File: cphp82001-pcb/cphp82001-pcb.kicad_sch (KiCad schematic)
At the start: 32 parts, among them J1 USB_B_Micro, J2 PAD+, J3 PAD-, Q1 2N7002, U1 BQ21040, U2 TLV75801, U3 MAX40203AUK, U4 TPS3808DBV, U6 NCP360SNT

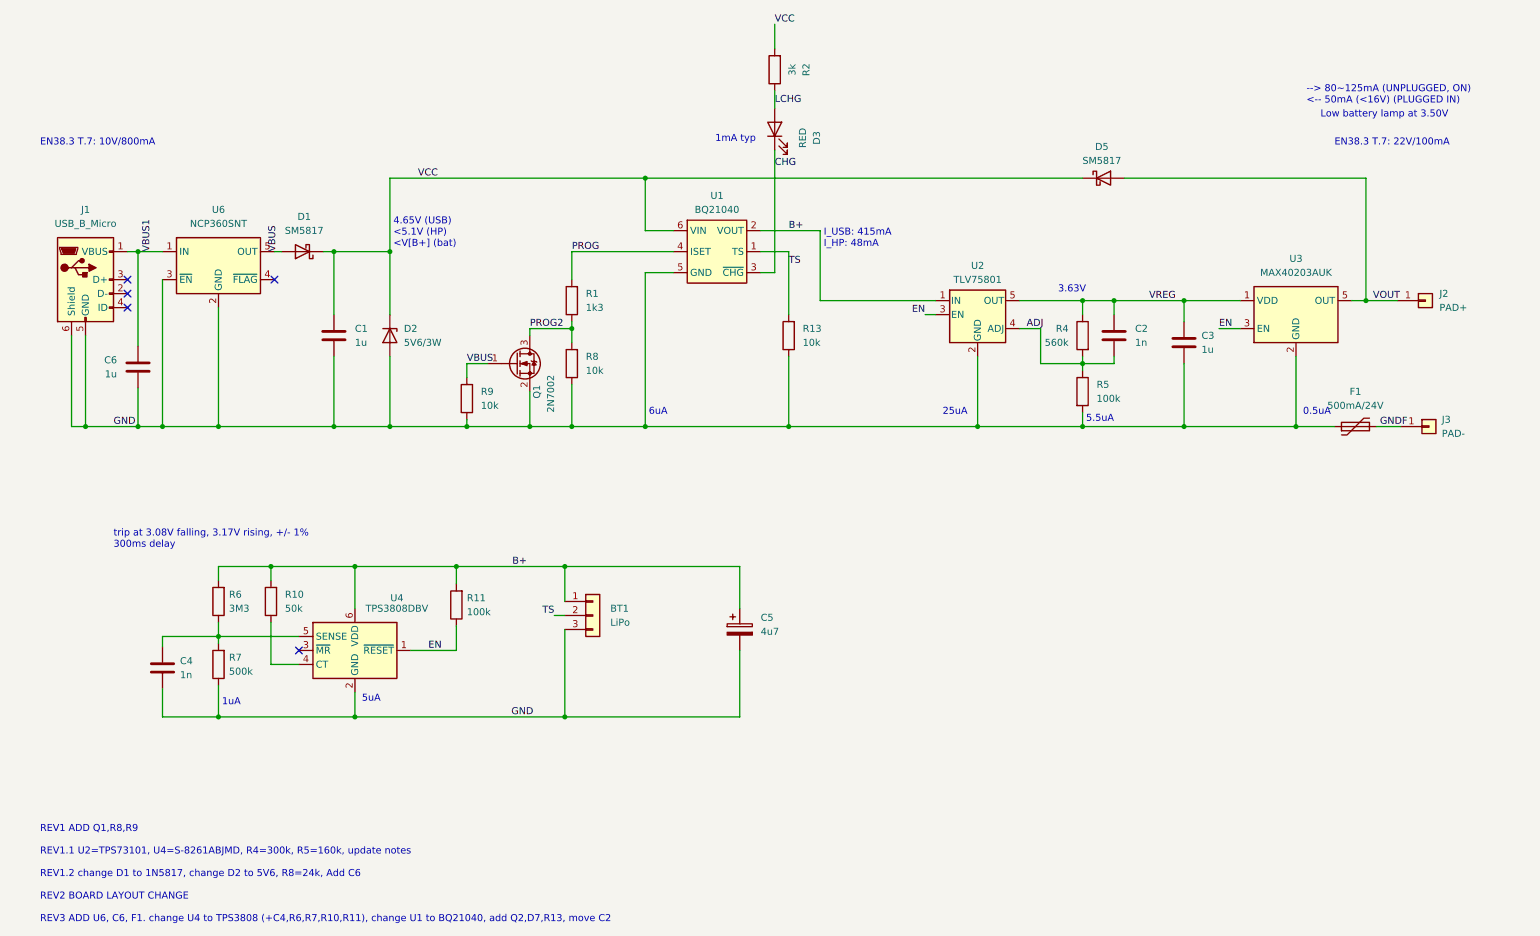
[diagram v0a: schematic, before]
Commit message: Update rev3
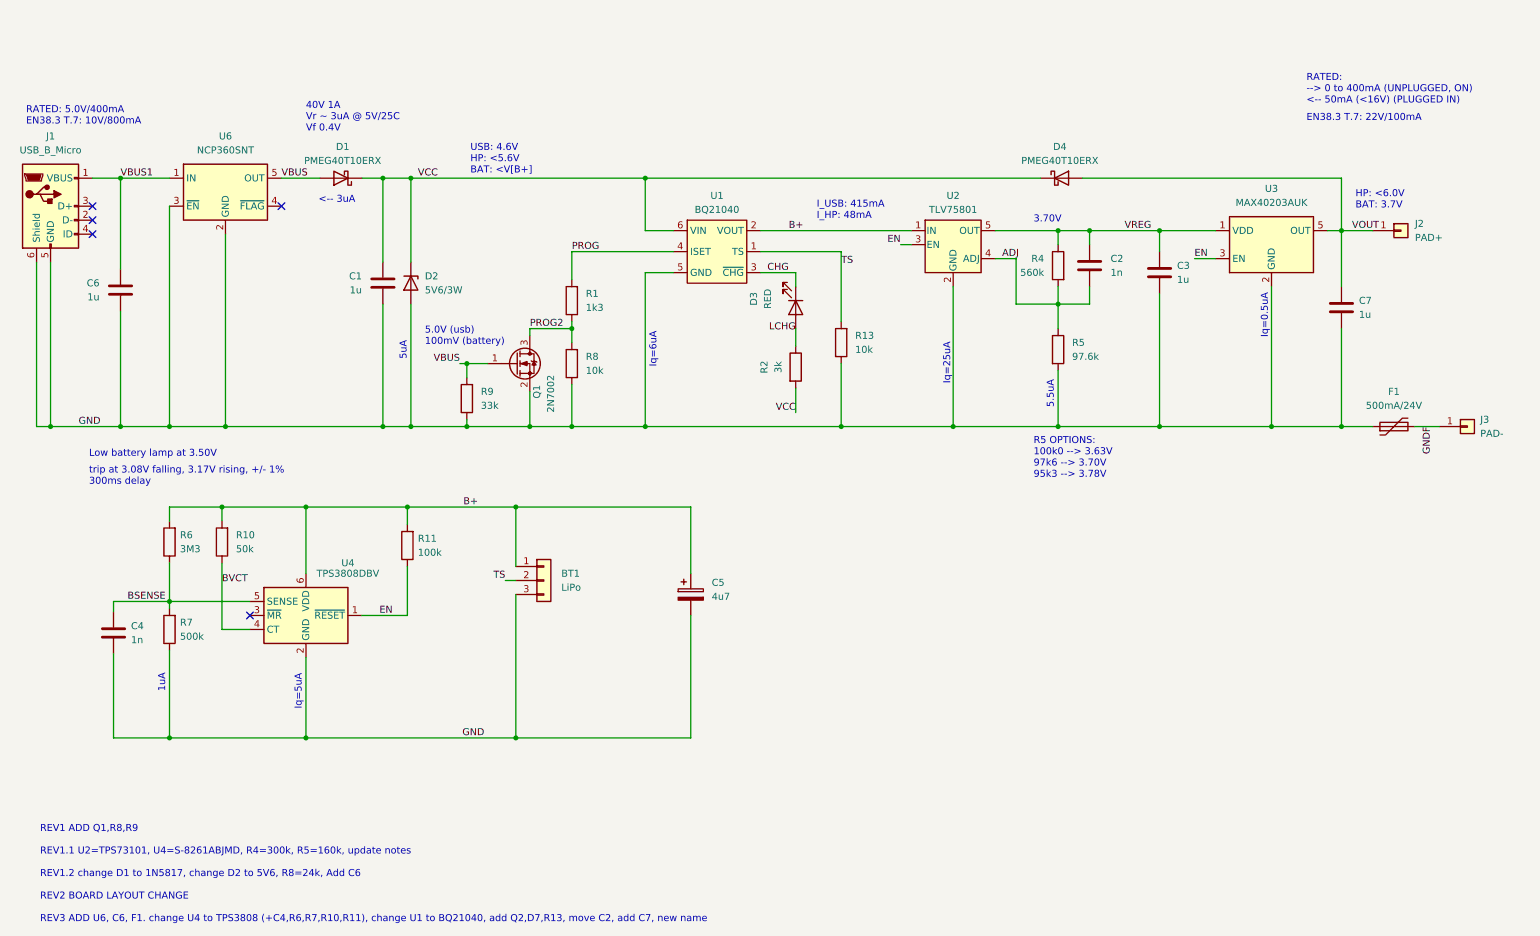
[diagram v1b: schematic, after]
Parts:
- removed D5: SM5817, Diode_SMD:D_SOD-123, symbol Diode:1N5819
- added C7: 1u, Capacitor_SMD:C_0805_2012Metric, symbol Device:C
- added D4: PMEG40T10ERX, Diode_SMD:D_SOD-123, symbol Diode:1N5819
- D1: value SM5817 -> PMEG40T10ERX
- R5: value 100k -> 97.6k
- R9: value 10k -> 33k
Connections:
- net GND: now also C7.2
- net VCC: now also D4.1 (K)
- net VOUT: now also C7.1, D4.2 (A)
- net BSENSE: now reaches C4.1, R6.1, R7.2, U4.5 (SENSE)
- net BVCT: now reaches R10.1, U4.4 (CT)
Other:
- note added: "3.70V"
- note added: "40V 1A Vr ~ 3uA @ 5V/25C Vf 0.4V"
- note added: "5.0V (usb) 100mV (battery)"
- note added: "<-- 3uA"
- note added: "HP: <6.0V BAT: 3.7V"
- note added: "Iq=0.5uA"
- note added: "Iq=25uA"
- note added: "Iq=5uA"
- note added: "Iq=6uA"
- note added: "R5 OPTIONS: 100k0 --> 3.63V 97k6 --> 3.70V 95k3 --> 3.78V"
- note added: "RATED: --> 0 to 400mA (UNPLUGGED, ON) <-- 50mA (<16V) (PLUGGED IN)"
- note added: "RATED: 5.0V/400mA EN38.3 T.7: 10V/800mA"
- note added: "REV1 ADD Q1,R8,R9 REV1.1 U2=TPS73101, U4=S-8261ABJMD, R4=300k, R5=160k, update notes REV1.2 change D1 to 1N5817, change D2 to 5V6, R8=24k, Add C6 REV2 BOARD LAYOUT CHANGE REV3 ADD U6, C6, F1. change U4 to TPS3808 (+C4,R6,R7,R10,R11), change U1 to BQ21040, add Q2,D7,R13, move C2, add C7, new name"
- note added: "USB: 4.6V HP: <5.6V BAT: <V[B+]"
- note removed: "--> 80~125mA (UNPLUGGED, ON) <-- 50mA (<16V) (PLUGGED IN)"
- note removed: "0.5uA"
- note removed: "1mA typ"
- note removed: "25uA"
- note removed: "3.63V"
- note removed: "4.65V (USB) <5.1V (HP) <V[B+] (bat)"
- note removed: "6uA"
- note removed: "EN38.3 T.7: 10V/800mA"
- note removed: "REV1 ADD Q1,R8,R9 REV1.1 U2=TPS73101, U4=S-8261ABJMD, R4=300k, R5=160k, update notes REV1.2 change D1 to 1N5817, change D2 to 5V6, R8=24k, Add C6 REV2 BOARD LAYOUT CHANGE REV3 ADD U6, C6, F1. change U4 to TPS3808 (+C4,R6,R7,R10,R11), change U1 to BQ21040, add Q2,D7,R13, move C2"
- company: GR -> calcpsu.com.au
- moved on the sheet: BT1, C1, C2, C3, C4, C5, C6, D1, D2, D3, F1, J1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
